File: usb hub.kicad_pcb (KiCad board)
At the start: 2 copper layers, 22 parts, among them J1 TYPE_C, U1 FE1.1s

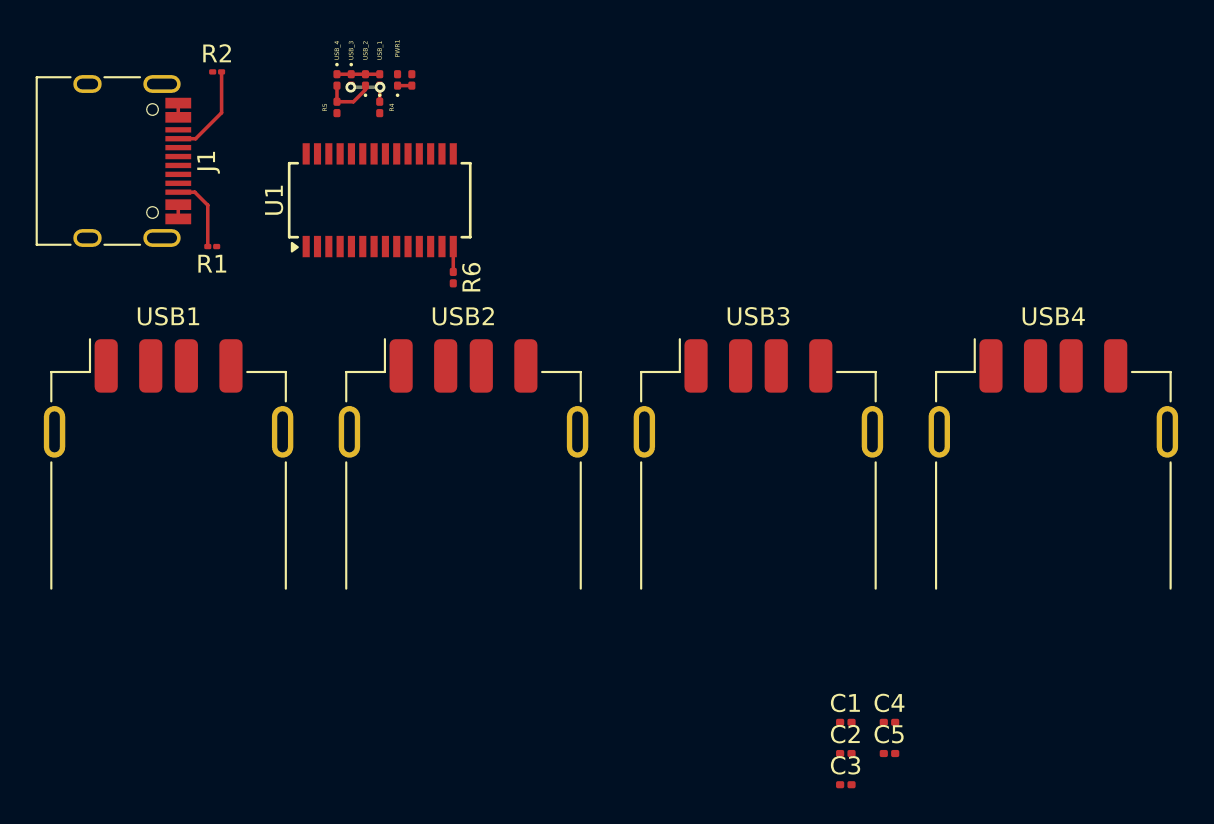
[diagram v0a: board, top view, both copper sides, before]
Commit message: all routes fixed AND placed parts
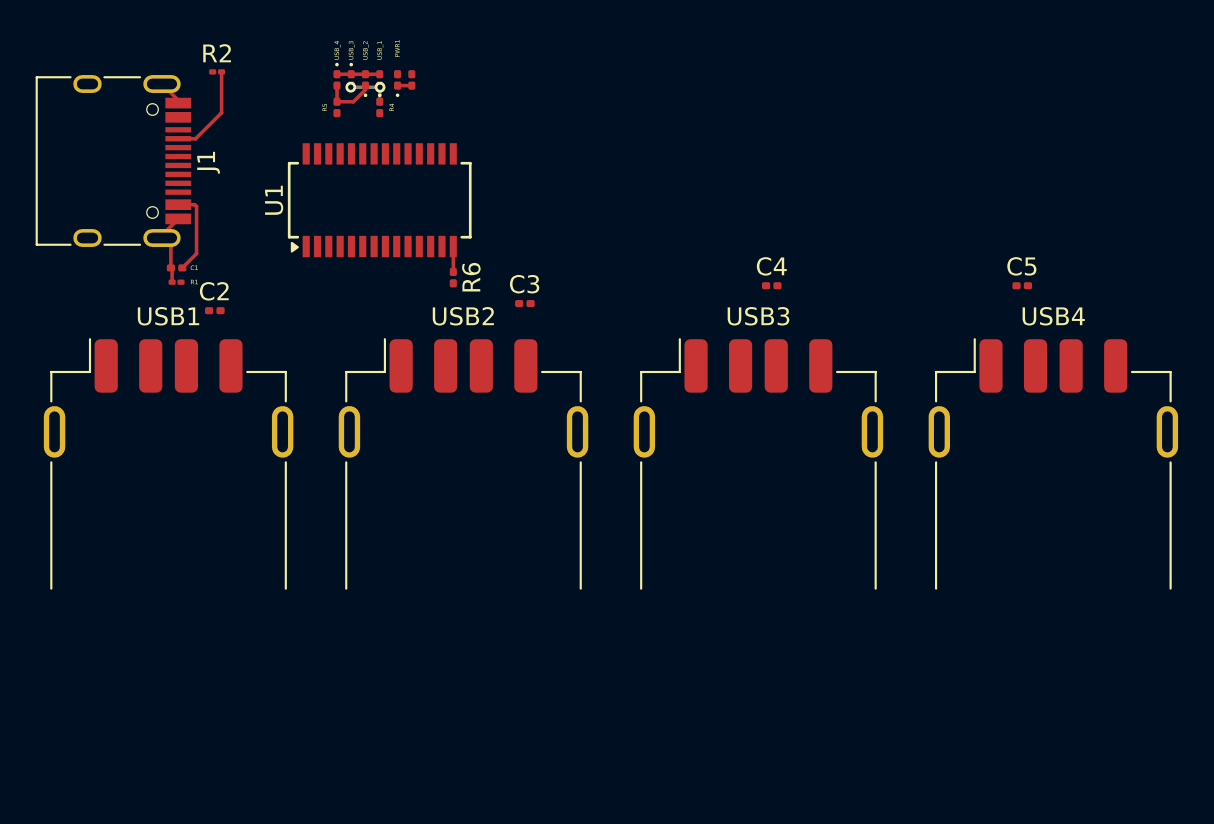
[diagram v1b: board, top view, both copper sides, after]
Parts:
- moved C1 45.4 mm to (125.2, 97.8)
- moved C2 43.3 mm to (127.3, 100.2)
- moved C3 32.5 mm to (144.7, 99.8)
- moved C5 27.3 mm to (172.7, 98.8)
- moved C4 25.4 mm to (158.6, 98.8)
- moved R1 2.83 mm to (125.2, 98.6), turned to 0 degrees
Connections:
- J1 pad A1: (no net) -> GNDREF
- J1 pad A12: (no net) -> GNDREF
- J1 pad A4: (no net) -> +5V
- J1 pad A9: (no net) -> +5V
- J1 pad B1: (no net) -> GNDREF
- J1 pad B12: (no net) -> GNDREF
- J1 pad B4: (no net) -> +5V
- J1 pad B9: (no net) -> +5V
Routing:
- net GNDREF: track 2.40 -> 8.01 mm
- net +5V: track 0.00 -> 4.85 mm
- net Net-(J1-CC2): track 4.28 -> 0.00 mm
- net (no net): track 1.60 -> 0.00 mm
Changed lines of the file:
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@@
 	(footprint "Resistor_SMD:R_01005_0402Metric"
 		(layer "F.Cu")
-		(at 127.2 96.6 180)
+		(at 125.2 98.6)
 		(descr "Resistor SMD 01005 (0402 Metric), square (rectangular) end terminal, IPC_7351 nominal, (Body size source: http://www.vishay.com/docs/20056/crcw01005e3.pdf), generated with kicad-footprint-generator")
 		(tags "resistor")
@@
 			(at 0 -1 360)
 			(layer "F.SilkS")
+			(hide yes)
 			(effects
 				(font
@@
 		)
 		(property "Footprint" "Resistor_SMD:R_01005_0402Metric"
-			(at 0 0 180)
+			(at 0 0 0)
 			(unlocked yes)
 			(layer "F.Fab")
@@
 		)
 		(property "Datasheet" ""
-			(at 0 0 180)
+			(at 0 0 0)
 			(unlocked yes)
 			(layer "F.Fab")
@@
 		)
 		(property "Description" "Resistor"
-			(at 0 0 180)
+			(at 0 0 0)
 			(unlocked yes)
 			(layer "F.Fab")
@@
 		(attr smd)
 		(fp_line
-			(start 0.6 0.3)
-			(end -0.6 0.3)
+			(start -0.6 -0.3)
+			(end 0.6 -0.3)
 			(stroke
 				(width 0.05)
@@
 		)
 		(fp_line
-			(start 0.6 -0.3)
-			(end 0.6 0.3)
+			(start -0.6 0.3)
+			(end -0.6 -0.3)
 			(stroke
 				(width 0.05)
@@
 		)
 		(fp_line
-			(start -0.6 0.3)
-			(end -0.6 -0.3)
+			(start 0.6 -0.3)
+			(end 0.6 0.3)
 			(stroke
 				(width 0.05)
@@
 		)
 		(fp_line
-			(start -0.6 -0.3)
-			(end 0.6 -0.3)
+			(start 0.6 0.3)
+			(end -0.6 0.3)
 			(stroke
 				(width 0.05)
@@
 		)
 		(fp_line
-			(start 0.2 0.1)
-			(end -0.2 0.1)
+			(start -0.2 -0.1)
+			(end 0.2 -0.1)
 			(stroke
 				(width 0.1)
@@
 		)
 		(fp_line
-			(start 0.2 -0.1)
-			(end 0.2 0.1)
+			(start -0.2 0.1)
+			(end -0.2 -0.1)
 			(stroke
 				(width 0.1)
@@
 		)
 		(fp_line
-			(start -0.2 0.1)
-			(end -0.2 -0.1)
+			(start 0.2 -0.1)
+			(end 0.2 0.1)
 			(stroke
 				(width 0.1)
@@
 		)
 		(fp_line
-			(start -0.2 -0.1)
-			(end 0.2 -0.1)
+			(start 0.2 0.1)
+			(end -0.2 0.1)
 			(stroke
 				(width 0.1)
@@
 		)
 		(fp_text user "${REFERENCE}"
-			(at 0 -0.62 360)
-			(layer "F.Fab")
+			(at 1 0 0)
+			(layer "F.SilkS")
 			(effects
 				(font
@@
 		)
 		(pad "" smd roundrect
-			(at -0.275 0 180)
+			(at -0.275 0)
 			(size 0.27 0.27)
 			(layers "F.Paste")
@@
 		)
 		(pad "" smd roundrect
-			(at 0.275 0 180)
+			(at 0.275 0)
 			(size 0.27 0.27)
 			(layers "F.Paste")
@@
 		)
 		(pad "1" smd roundrect
-			(at -0.25 0 180)
+			(at -0.25 0)
 			(size 0.4 0.3)
 			(layers "F.Cu" "F.Mask")
@@
 		)
 		(pad "2" smd roundrect
-			(at 0.25 0 180)
+			(at 0.25 0)
 			(size 0.4 0.3)
 			(layers "F.Cu" "F.Mask")
@@
 	(footprint "Capacitor_SMD:C_0201_0603Metric"
 		(layer "F.Cu")
-		(at 162.755 126.8)
+		(at 144.745 99.8)
 		(descr "Capacitor SMD 0201 (0603 Metric), square (rectangular) end terminal, IPC_7351 nominal, (Body size source: https://www.vishay.com/docs/20052/crcw0201e3.pdf), generated with kicad-footprint-generator")
 		(tags "capacitor")
@@
 	(footprint "Capacitor_SMD:C_0201_0603Metric"
 		(layer "F.Cu")
-		(at 165.205 123.3)
+		(at 158.6 98.8)
 		(descr "Capacitor SMD 0201 (0603 Metric), square (rectangular) end terminal, IPC_7351 nominal, (Body size source: https://www.vishay.com/docs/20052/crcw0201e3.pdf), generated with kicad-footprint-generator")
 		(tags "capacitor")
@@
 	(footprint "Capacitor_SMD:C_0201_0603Metric"
 		(layer "F.Cu")
-		(at 162.755 123.3)
+		(at 125.2 97.8)
 		(descr "Capacitor SMD 0201 (0603 Metric), square (rectangular) end terminal, IPC_7351 nominal, (Body size source: https://www.vishay.com/docs/20052/crcw0201e3.pdf), generated with kicad-footprint-generator")
 		(tags "capacitor")
@@
 			(at 0 -1.05 0)
 			(layer "F.SilkS")
+			(hide yes)
 			(effects
 				(font
@@
 			(at 0 1.05 0)
 			(layer "F.Fab")
+			(hide yes)
 			(effects
 				(font
@@
 		)
 		(fp_text user "${REFERENCE}"
-			(at 0 -0.68 0)
-			(layer "F.Fab")
+			(at 1 0 0)
+			(layer "F.SilkS")
 			(effects
 				(font
@@
 			(size 0.6 1.45)
 			(layers "F.Cu" "F.Paste" "F.Mask")
+			(net 21 "GNDREF")
+			(pinfunction "GND")
+			(pintype "power_in")
 		)
 		(pad "A4" smd rect
@@
 			(size 0.6 1.45)
 			(layers "F.Cu" "F.Paste" "F.Mask")
+			(net 14 "+5V")
+			(pinfunction "VBUS")
+			(pintype "power_in")
 		)
 		(pad "A5" smd rect
@@
 			(size 0.6 1.45)
 			(layers "F.Cu" "F.Paste" "F.Mask")
+			(net 14 "+5V")
+			(pinfunction "VBUS")
+			(pintype "power_in")
 		)
 		(pad "A12" smd rect
@@
 			(size 0.6 1.45)
 			(layers "F.Cu" "F.Paste" "F.Mask")
+			(net 21 "GNDREF")
+			(pinfunction "GND")
+			(pintype "power_in")
 		)
 		(pad "B1" smd rect
@@
 			(size 0.6 1.45)
 			(layers "F.Cu" "F.Paste" "F.Mask")
+			(net 21 "GNDREF")
+			(pinfunction "GND")
+			(pintype "power_in")
 		)
 		(pad "B4" smd rect
@@
 			(size 0.6 1.45)
 			(layers "F.Cu" "F.Paste" "F.Mask")
+			(net 14 "+5V")
+			(pinfunction "VBUS")
+			(pintype "power_in")
 		)
 		(pad "B5" smd rect
@@
 			(size 0.6 1.45)
 			(layers "F.Cu" "F.Paste" "F.Mask")
+			(net 14 "+5V")
+			(pinfunction "VBUS")
+			(pintype "power_in")
 		)
 		(pad "B12" smd rect
@@
 			(size 0.6 1.45)
 			(layers "F.Cu" "F.Paste" "F.Mask")
+			(net 21 "GNDREF")
+			(pinfunction "GND")
+			(pintype "power_in")
 		)
 		(pad "S1" thru_hole oval
@@
 	(footprint "Capacitor_SMD:C_0201_0603Metric"
 		(layer "F.Cu")
-		(at 162.755 125.05)
+		(at 127.345 100.2)
 		(descr "Capacitor SMD 0201 (0603 Metric), square (rectangular) end terminal, IPC_7351 nominal, (Body size source: https://www.vishay.com/docs/20052/crcw0201e3.pdf), generated with kicad-footprint-generator")
 		(tags "capacitor")
@@
 	(footprint "Capacitor_SMD:C_0201_0603Metric"
 		(layer "F.Cu")
-		(at 165.205 125.05)
+		(at 172.655 98.8)
 		(descr "Capacitor SMD 0201 (0603 Metric), square (rectangular) end terminal, IPC_7351 nominal, (Body size source: https://www.vishay.com/docs/20052/crcw0201e3.pdf), generated with kicad-footprint-generator")
 		(tags "capacitor")
@@
 	)
 	(segment
-		(start 125.295 89.35)
-		(end 125.295 88.55)
+		(start 126.22 94.25)
+		(end 125.295 94.25)
 		(width 0.2)
 		(layer "F.Cu")
-		(net 0)
+		(net 14)
 	)
 	(segment
-		(start 125.295 94.25)
-		(end 125.295 95.05)
+		(start 126.32 97)
+		(end 126.32 94.35)
+		(width 0.2)
+		(layer "F.Cu")
+		(net 14)
+	)
+	(segment
+		(start 126.32 94.35)
+		(end 126.22 94.25)
+		(width 0.2)
+		(layer "F.Cu")
+		(net 14)
+	)
+	(segment
+		(start 125.52 97.8)
+		(end 126.32 97)
 		(width 0.2)
 		(layer "F.Cu")
-		(net 0)
+		(net 14)
 	)
 	(segment
@@
 	)
 	(segment
-		(start 126.95 94.28)
-		(end 126.22 93.55)
+		(start 124.38 96.12)
+		(end 124.38 95.965002)
 		(width 0.2)
 		(layer "F.Cu")
-		(net 24)
+		(net 21)
 	)
 	(segment
-		(start 126.95 96.6)
-		(end 126.95 94.28)
+		(start 125.295 95.050002)
+		(end 125.295 95.05)
 		(width 0.2)
 		(layer "F.Cu")
-		(net 24)
+		(net 21)
 	)
 	(segment
-		(start 126.22 93.55)
-		(end 125.295 93.55)
+		(start 124.95 98.6)
+		(end 124.95 97.87)
 		(width 0.2)
 		(layer "F.Cu")
-		(net 24)
+		(net 21)
+	)
+	(segment
+		(start 124.88 96.62)
+		(end 124.38 96.12)
+		(width 0.2)
+		(layer "F.Cu")
+		(net 21)
+	)
+	(segment
+		(start 125.295 88.55)
+		(end 125.295 88.395)
+		(width 0.2)
+		(layer "F.Cu")
+		(net 21)
+	)
+	(segment
+		(start 125.295 88.395)
+		(end 124.38 87.48)
+		(width 0.2)
+		(layer "F.Cu")
+		(net 21)
+	)
+	(segment
+		(start 124.95 97.87)
+		(end 124.88 97.8)
+		(width 0.2)
+		(layer "F.Cu")
+		(net 21)
+	)
+	(segment
+		(start 124.88 97.8)
+		(end 124.88 96.62)
+		(width 0.2)
+		(layer "F.Cu")
+		(net 21)
+	)
+	(segment
+		(start 124.38 95.965002)
+		(end 125.295 95.050002)
+		(width 0.2)
+		(layer "F.Cu")
+		(net 21)
 	)
 	(segment
